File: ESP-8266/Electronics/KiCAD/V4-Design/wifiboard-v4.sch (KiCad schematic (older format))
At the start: 37 parts, among them IC1 78033AF, J1 PWR, J10 Conn_01x01_Male, J2 thermistor, J3 Aux1, J4 Aux2, J5 USB-3V3, J6 PROG, J7 OUT, J8 mains, J9 Conn_01x01_Male, K1 CPC1966Y, Q1 FDD8870, SW1 reset, U1 ESP-12E

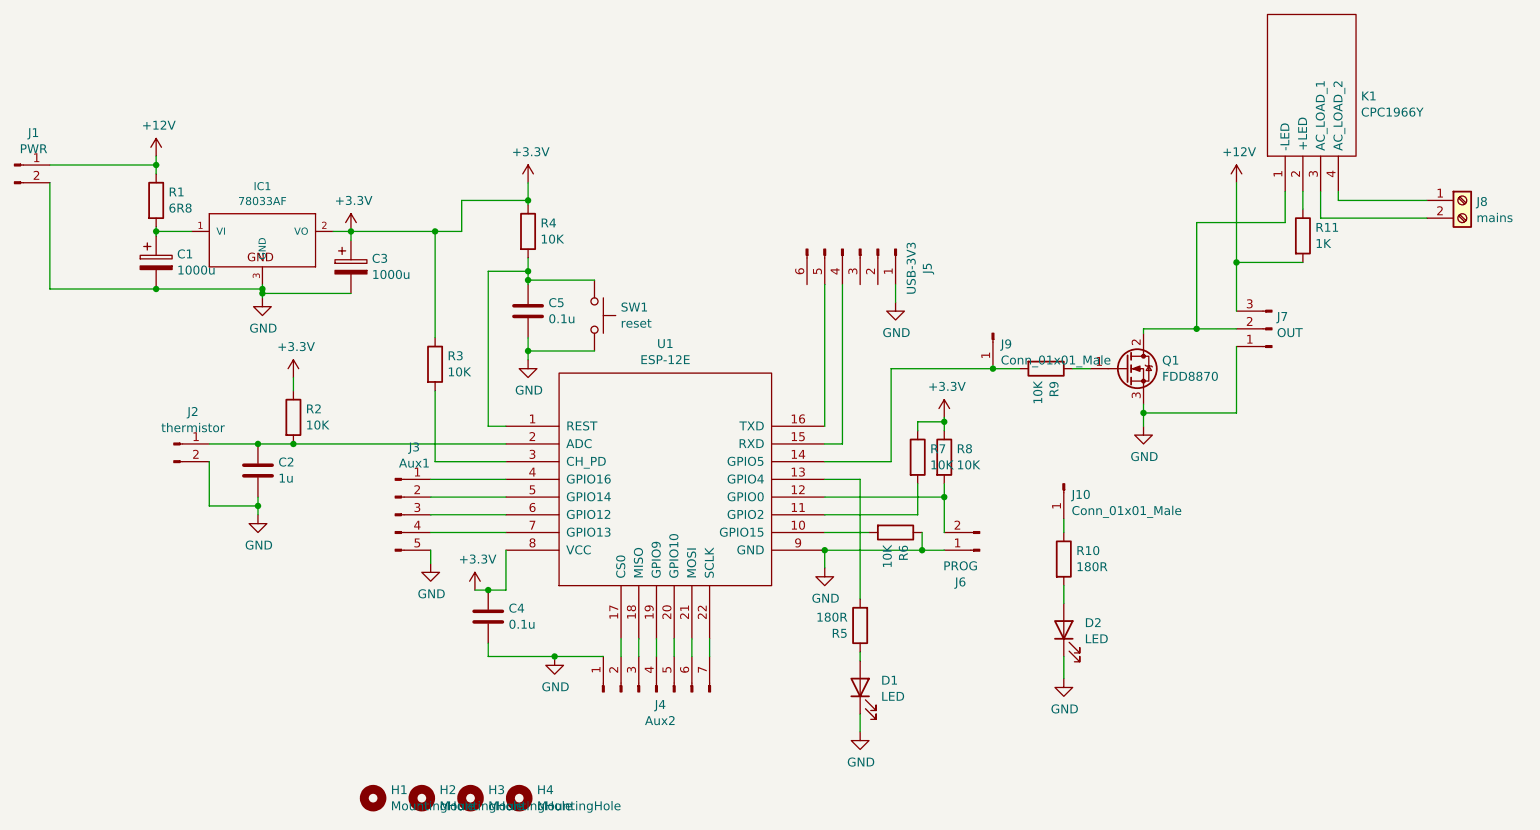
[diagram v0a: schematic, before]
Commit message: SB & AB PCB layout
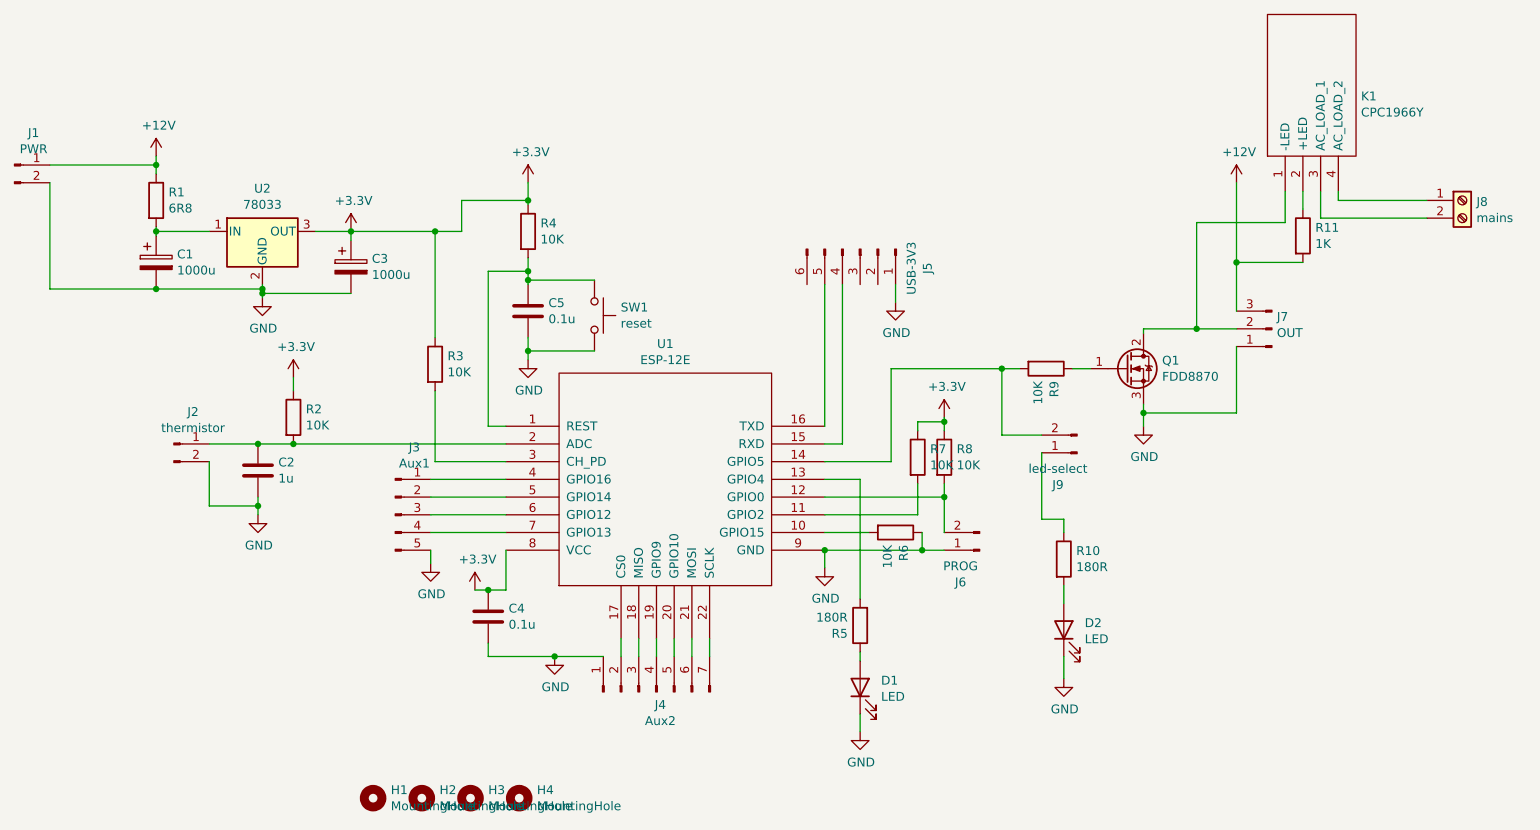
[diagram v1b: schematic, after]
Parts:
- removed IC1: 78033AF, Package_TO_SOT_SMD:TO-252-2, symbol adafruit-new:7805DT
- removed J10, J9: Conn_01x01_Male, Connector_PinHeader_2.54mm:PinHeader_1x01_P2.54mm_Vertical, symbol Connector:Conn_01x01_Male
- added J9: led-select, Connector_PinHeader_2.54mm:PinHeader_1x02_P2.54mm_Vertical, symbol Connector:Conn_01x02_Male
- added U2: 78033, Package_TO_SOT_SMD:TO-252-2, symbol Regulator_Linear:L7805
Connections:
- net +3V3: now also U2.3 (OUT)
- net GND: now also U2.2 (GND)
- net at R9.2, U1.14 (GPIO5): now also J9.2 (Pin_2)
- net at C1.1, R1.2: now also U2.1 (IN)
- net at R10.1: now also J9.1 (Pin_1)
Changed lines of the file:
@@
 	4000 3575 4000 3600
-$Comp
-L adafruit-new:7805DT IC1
-U 1 1 61F84DB3
-P 2500 3300
-F 0 "IC1" H 2500 3554 45  0000 C CNN
-F 1 "78033AF" H 2500 3470 45  0000 C CNN
-F 2 "Package_TO_SOT_SMD:TO-252-2" H 2530 3450 20  0001 C CNN
-F 3 "" H 2500 3300 50  0001 C CNN
-	1    2500 3300
-	1    0    0    -1
-$EndComp
 $Comp
 L Device:R R1
@@
 $EndComp
 Wire Wire Line
-	2100 3300 1900 3300
-Wire Wire Line
 	1900 3300 1900 3275
 $Comp
@@
 	1    0    0    -1
 $EndComp
-Wire Wire Line
-	2500 3600 2500 3625
 $Comp
 L power:+12V #PWR0110
@@
 Wire Wire Line
 	1300 3625 1900 3625
-Connection ~ 2500 3625
-Wire Wire Line
-	2500 3625 2500 3650
 $Comp
 L power:+3.3V #PWR0111
@@
 	1    0    0    -1
 $EndComp
-Wire Wire Line
-	2900 3300 3000 3300
 $Comp
 L Device:CP C1
@@
 	1    0    0    -1
 $EndComp
-Connection ~ 1900 3625
-Wire Wire Line
-	1900 3625 2500 3625
 Wire Wire Line
 	1900 3300 1900 3325
 Connection ~ 1900 3300
-Wire Wire Line
-	3000 3650 2500 3650
-Connection ~ 2500 3650
-Wire Wire Line
-	2500 3650 2500 3675
 Wire Wire Line
 	3000 3350 3000 3300
@@
 Wire Wire Line
 	5675 4600 6050 4600
-Wire Wire Line
-	6050 4075 6625 4075
 $Comp
 L Device:R R9
@@
 Wire Wire Line
 	7025 5700 7025 5825
-$Comp
-L Connector:Conn_01x01_Male J10
-U 1 1 62042A4C
-P 7025 4725
-F 0 "J10" V 7087 4769 50  0000 L CNN
-F 1 "Conn_01x01_Male" V 7178 4769 50  0000 L CNN
-F 2 "Connector_PinHeader_2.54mm:PinHeader_1x01_P2.54mm_Vertical" H 7025 4725 50  0001 C CNN
-F 3 "~" H 7025 4725 50  0001 C CNN
-	1    7025 4725
-	0    1    1    0
-$EndComp
 Wire Wire Line
 	7025 4925 7025 5000
 $Comp
-L Connector:Conn_01x01_Male J9
-U 1 1 62057289
-P 6625 3875
-F 0 "J9" V 6687 3919 50  0000 L CNN
-F 1 "Conn_01x01_Male" V 6778 3919 50  0000 L CNN
-F 2 "Connector_PinHeader_2.54mm:PinHeader_1x01_P2.54mm_Vertical" H 6625 3875 50  0001 C CNN
-F 3 "~" H 6625 3875 50  0001 C CNN
-	1    6625 3875
-	0    1    1    0
-$EndComp
-Connection ~ 6625 4075
-Wire Wire Line
-	6625 4075 6775 4075
+L Connector:Conn_01x02_Male J9
+U 1 1 61FC195B
+P 7100 4550
+F 0 "J9" H 7208 4731 50  0000 C CNN
+F 1 "led-select" H 7208 4640 50  0000 C CNN
+F 2 "Connector_PinHeader_2.54mm:PinHeader_1x02_P2.54mm_Vertical" H 7100 4550 50  0001 C CNN
+F 3 "~" H 7100 4550 50  0001 C CNN
+	1    7100 4550
+	-1   0    0    1
+$EndComp
+Wire Wire Line
+	6050 4075 6675 4075
+Wire Wire Line
+	6675 4075 6675 4450
+Wire Wire Line
+	6675 4450 6900 4450
+Connection ~ 6675 4075
+Wire Wire Line
+	6675 4075 6775 4075
+Wire Wire Line
+	7025 4925 6900 4925
+Wire Wire Line
+	6900 4925 6900 4550
+$Comp
+L Regulator_Linear:L7805 U2
+U 1 1 61FDBAF2
+P 2500 3300
+F 0 "U2" H 2500 3542 50  0000 C CNN
+F 1 "78033" H 2500 3451 50  0000 C CNN
+F 2 "Package_TO_SOT_SMD:TO-252-2" H 2525 3150 50  0001 L CIN
+F 3 "http://www.st.com/content/ccc/resource/technical/document/datasheet/41/4f/b3/b0/12/d4/47/88/CD00000444.pdf/files/CD00000444.pdf/jcr:content/translations/en.CD00000444.pdf" H 2500 3250 50  0001 C CNN
+	1    2500 3300
+	1    0    0    -1
+$EndComp
+Wire Wire Line
+	1900 3300 2200 3300
+Wire Wire Line
+	2800 3300 3000 3300
+Wire Wire Line
+	2500 3600 2500 3625
+Wire Wire Line
+	3000 3650 2500 3650
+Connection ~ 2500 3650
+Wire Wire Line
+	2500 3650 2500 3675
+Wire Wire Line
+	1900 3625 2500 3625
+Connection ~ 1900 3625
+Connection ~ 2500 3625
+Wire Wire Line
+	2500 3625 2500 3650
 $EndSCHEMATC

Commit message: PCB sent for trial production.
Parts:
- added JP1: SolderJumper_2_Bridged, Jumper:SolderJumper-2_P1.3mm_Bridged_RoundedPad1.0x1.5mm, symbol Jumper:SolderJumper_2_Bridged
- K1: symbol cpc1966y:CPC1966Y -> wifiboard-v4-rescue:CPC1966Y-cpc1966y
- U1: symbol esp-8266:ESP-12E -> wifiboard-v4-rescue:ESP-12E-esp-8266
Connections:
- net at J9.2 (Pin_2), R9.2, U1.14 (GPIO5): now also JP1.1 (A)
- net at J9.1 (Pin_1), R10.1: now also JP1.2 (B)
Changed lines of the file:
@@
 $EndComp
 $Comp
-L esp-8266:ESP-12E U1
+L wifiboard-v4-rescue:ESP-12E-esp-8266 U1
 U 1 1 61F7D88E
 P 4775 4700
@@
 	7475 4325 7475 4400
 $Comp
-L cpc1966y:CPC1966Y K1
+L wifiboard-v4-rescue:CPC1966Y-cpc1966y K1
 U 1 1 61FAC409
 P 8275 3075
@@
 	6675 4075 6675 4450
 Wire Wire Line
-	6675 4450 6900 4450
+	6675 4450 6725 4450
 Connection ~ 6675 4075
 Wire Wire Line
@@
 	7025 4925 6900 4925
 Wire Wire Line
-	6900 4925 6900 4550
+	6900 4925 6900 4750
 $Comp
 L Regulator_Linear:L7805 U2
@@
 Wire Wire Line
 	2500 3625 2500 3650
+$Comp
+L Jumper:SolderJumper_2_Bridged JP1
+U 1 1 61FD9520
+P 6725 4600
+F 0 "JP1" V 6679 4668 50  0000 L CNN
+F 1 "SolderJumper_2_Bridged" V 6770 4668 50  0000 L CNN
+F 2 "Jumper:SolderJumper-2_P1.3mm_Bridged_RoundedPad1.0x1.5mm" H 6725 4600 50  0001 C CNN
+F 3 "~" H 6725 4600 50  0001 C CNN
+	1    6725 4600
+	0    1    1    0
+$EndComp
+Connection ~ 6725 4450
+Wire Wire Line
+	6725 4450 6900 4450
+Wire Wire Line
+	6725 4750 6900 4750
+Connection ~ 6900 4750
+Wire Wire Line
+	6900 4750 6900 4550
 $EndSCHEMATC
